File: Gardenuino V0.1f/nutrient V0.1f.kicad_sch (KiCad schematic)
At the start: 85 parts, among them J1 Conn_01x04_Male, J2 Conn_01x04_Female, J3 Conn_01x04_Male, J4 Conn_01x04_Male, J5 Conn_01x04_Female, J6 Conn_01x04_Male, J7 Conn_01x03_Male, J8 Conn_01x03_Male, J9 Conn_01x01_Male, P1 SolderJumper_2_Open, P2 SolderJumper_2_Bridged, P3 SolderJumper_2_Bridged, Q1 Q_NMOS_DGS, Q10 Q_NMOS_DGS, Q2 Q_NMOS_DGS, Q3 Q_NMOS_DGS, Q4 Q_NMOS_DGS, Q5 Q_NMOS_DGS, Q6 Q_NMOS_DGS, Q7 Q_NMOS_DGS, Q8 2N3904, U1 23LC512, U2 DS1307+, Y1 Crystal_Small

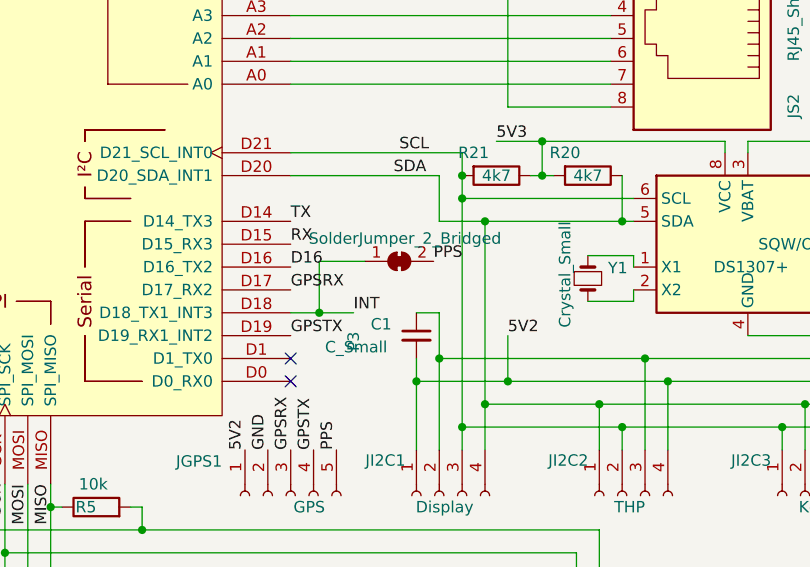
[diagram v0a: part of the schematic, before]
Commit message: SpectDrone Development
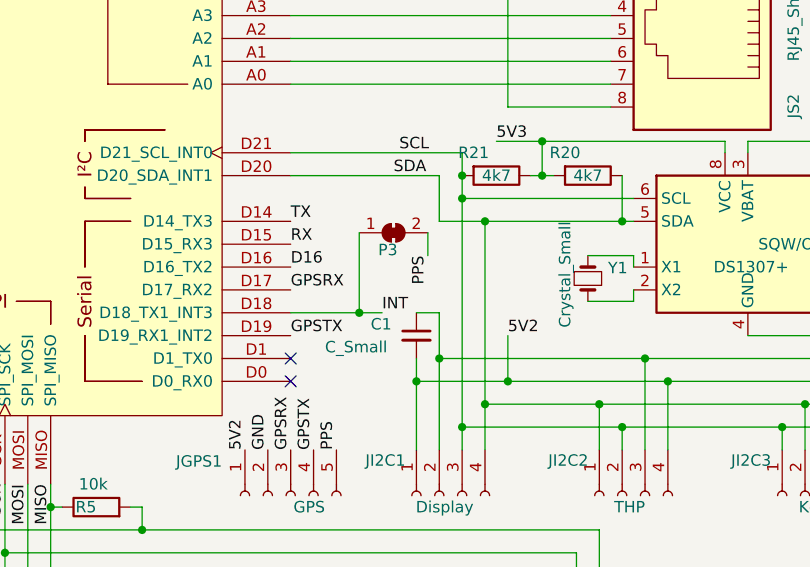
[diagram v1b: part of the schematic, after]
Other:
- moved on the sheet: P3
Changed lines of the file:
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@@
   (junction (at 222.25 102.87) (diameter 0) (color 0 0 0 0)
   )
+  (junction (at 210.82 118.11) (diameter 0) (color 0 0 0 0)
+  )
   (junction (at 134.62 133.35) (diameter 0) (color 0 0 0 0)
   )
@@
   )
   (junction (at 129.54 105.41) (diameter 0) (color 0 0 0 0)
-  )
-  (junction (at 206.375 118.11) (diameter 0) (color 0 0 0 0)
   )
   (junction (at 100.33 85.09) (diameter 0) (color 0 0 0 0)
@@
     (stroke (width 0) (type default) (color 0 0 0 0))
   )
-  (wire (pts (xy 206.375 112.395) (xy 211.455 112.395))
-    (stroke (width 0) (type default) (color 0 0 0 0))
-  )
   (wire (pts (xy 238.76 67.31) (xy 229.87 67.31))
     (stroke (width 0) (type default) (color 0 0 0 0))
@@
     (stroke (width 0) (type default) (color 0 0 0 0))
   )
+  (wire (pts (xy 210.82 118.11) (xy 213.36 118.11))
+    (stroke (width 0) (type default) (color 0 0 0 0))
+  )
   (wire (pts (xy 43.18 118.11) (xy 43.18 142.24))
     (stroke (width 0) (type default) (color 0 0 0 0))
   )
-  (wire (pts (xy 206.375 118.11) (xy 210.185 118.11))
-    (stroke (width 0) (type default) (color 0 0 0 0))
-  )
   (wire (pts (xy 176.53 139.7) (xy 176.53 137.16))
     (stroke (width 0) (type default) (color 0 0 0 0))
@@
     (stroke (width 0) (type default) (color 0 0 0 0))
   )
-  (wire (pts (xy 203.2 118.11) (xy 206.375 118.11))
+  (wire (pts (xy 203.2 118.11) (xy 210.82 118.11))
     (stroke (width 0) (type default) (color 0 0 0 0))
   )
@@
     (stroke (width 0) (type default) (color 0 0 0 0))
   )
-  (wire (pts (xy 206.375 118.11) (xy 206.375 112.395))
+  (wire (pts (xy 210.82 109.22) (xy 210.82 118.11))
     (stroke (width 0) (type default) (color 0 0 0 0))
   )
@@
     (stroke (width 0) (type default) (color 0 0 0 0))
   )
+  (wire (pts (xy 218.44 111.76) (xy 218.44 109.22))
+    (stroke (width 0) (type default) (color 0 0 0 0))
+  )
   (wire (pts (xy 265.43 125.73) (xy 266.7 125.73))
     (stroke (width 0) (type default) (color 0 0 0 0))
@@
     (effects (font (size 1.27 1.27)) (justify right bottom))
   )
-  (label "PPS" (at 219.075 112.395 0)
-    (effects (font (size 1.27 1.27)) (justify left bottom))
+  (label "PPS" (at 218.44 111.76 270)
+    (effects (font (size 1.27 1.27)) (justify right bottom))
   )
   (label "D13" (at 133.35 97.79 180)
@@
     (effects (font (size 1.27 1.27)) (justify right bottom))
   )
-  (label "INT" (at 210.185 118.11 0)
+  (label "INT" (at 213.36 118.11 0)
     (effects (font (size 1.27 1.27)) (justify left bottom))
   )
@@
     (pin "2")
   )
-  (symbol (lib_id "Jumper:SolderJumper_2_Bridged") (at 215.265 112.395 0) (unit 1)
-    (in_bom yes) (on_board yes)
-    (property "Reference" "P3" (id 0) (at 210.185 121.285 90))
-    (property "Value" "SolderJumper_2_Bridged" (id 1) (at 215.9 109.855 0))
-    (property "Footprint" "Library:SolderJumper-2_P1.3mm_Bridged2Bar_RoundedPad1.0x1.5mm_narrow" (id 2) (at 215.265 112.395 0)
-      (effects (font (size 1.27 1.27)) hide)
-    )
-    (property "Datasheet" "~" (id 3) (at 215.265 112.395 0)
-      (effects (font (size 1.27 1.27)) hide)
-    )
+  (symbol (lib_id "Jumper:SolderJumper_2_Bridged") (at 214.63 109.22 0) (unit 1)
+    (in_bom yes) (on_board yes)
+    (property "Reference" "P3" (id 0) (at 213.995 111.125 0))
+    (property "Value" "SolderJumper_2_Bridged" (id 1) (at 215.265 106.68 0)
+      (effects (font (size 1.27 1.27)) hide)
+    )
+    (property "Footprint" "Library:SolderJumper-2_P1.3mm_Bridged2Bar_RoundedPad1.0x1.5mm_narrow" (id 2) (at 214.63 109.22 0)
+      (effects (font (size 1.27 1.27)) hide)
+    )
+    (property "Datasheet" "~" (id 3) (at 214.63 109.22 0)
+      (effects (font (size 1.27 1.27)) hide)
+    )
